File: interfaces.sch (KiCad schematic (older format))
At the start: 11 parts

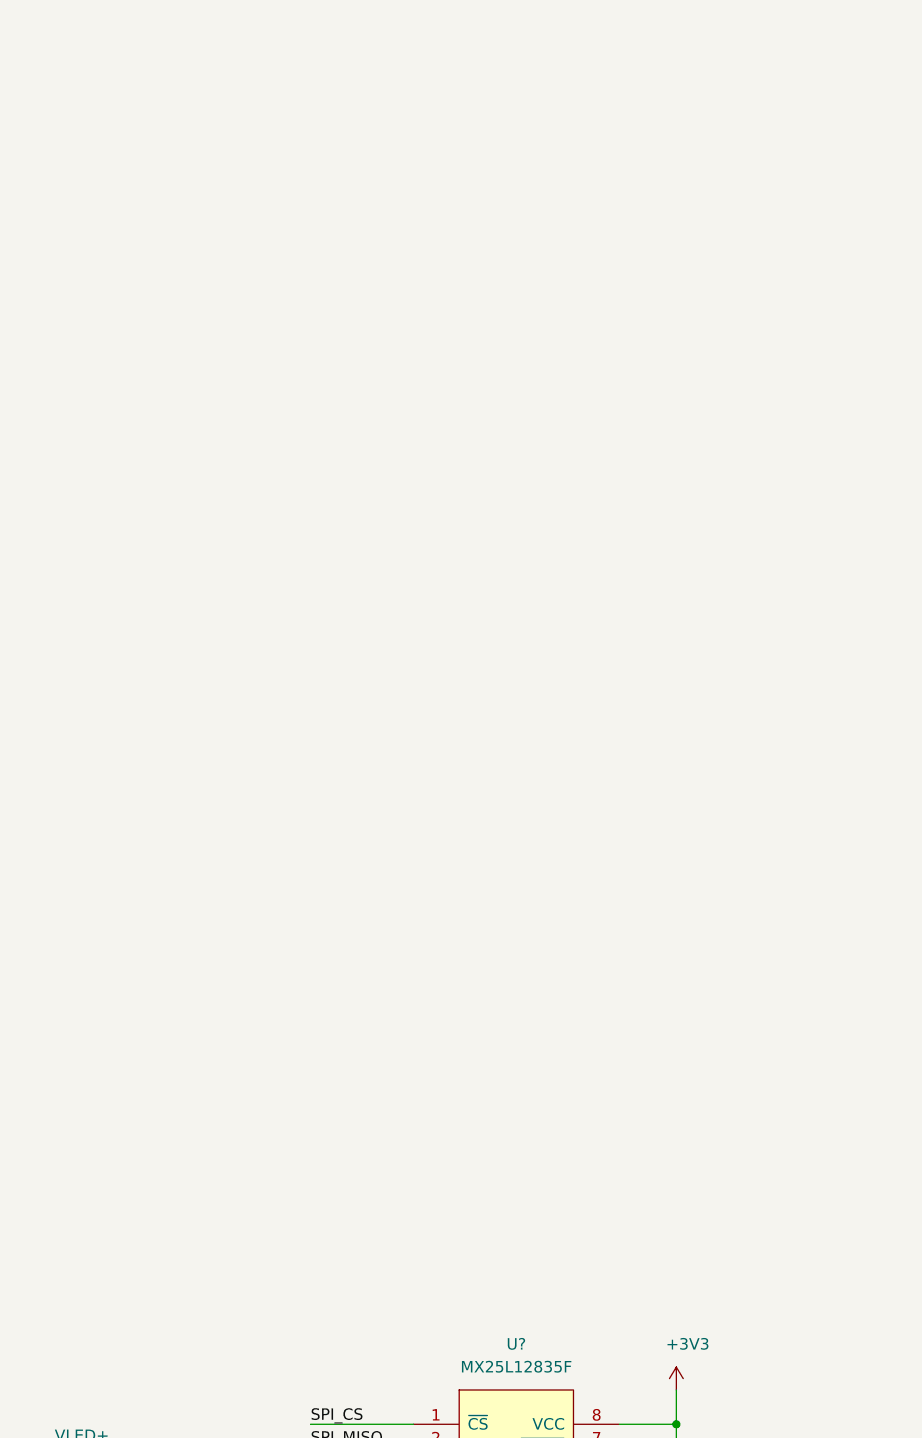
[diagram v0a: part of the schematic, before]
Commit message: update,
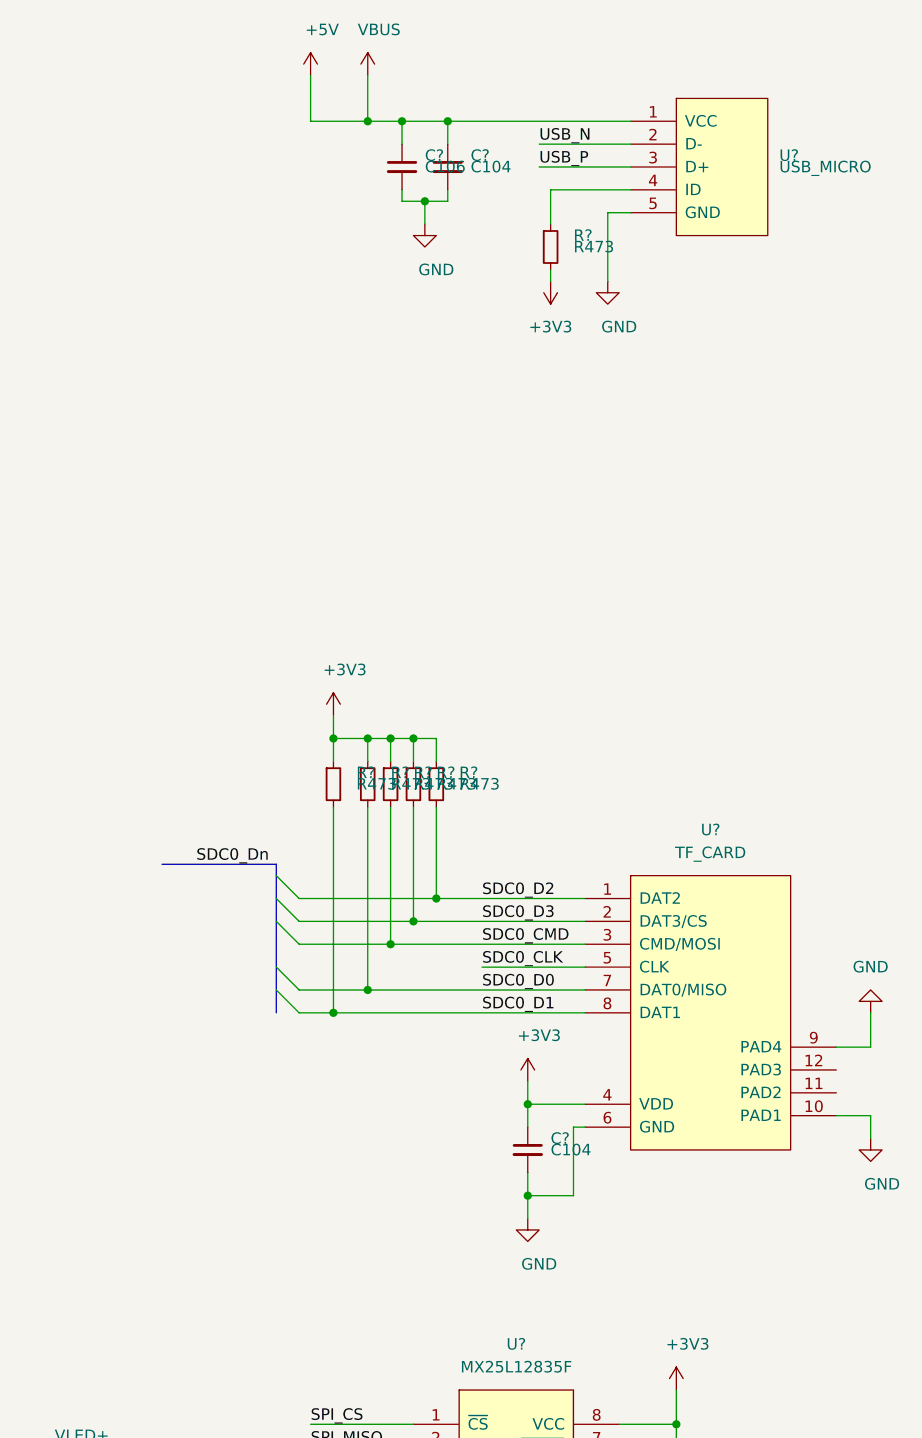
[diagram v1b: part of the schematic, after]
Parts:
- added C? (x2): C104, symbol taobao-c:C104
- added C?: C106, symbol taobao-c:C106
- added R? (x6): R473, symbol taobao-r:R473
- added U?: TF_CARD, symbol taobao-components:TF_CARD
- added U?: USB_MICRO, symbol taobao-components:USB_MICRO
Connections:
- net labels added: SDC0_CLK, SDC0_CMD, SDC0_D0, SDC0_D1, SDC0_D2, SDC0_D3, SDC0_Dn, USB_N, USB_P, VBUS
- wire segments 108 -> 166

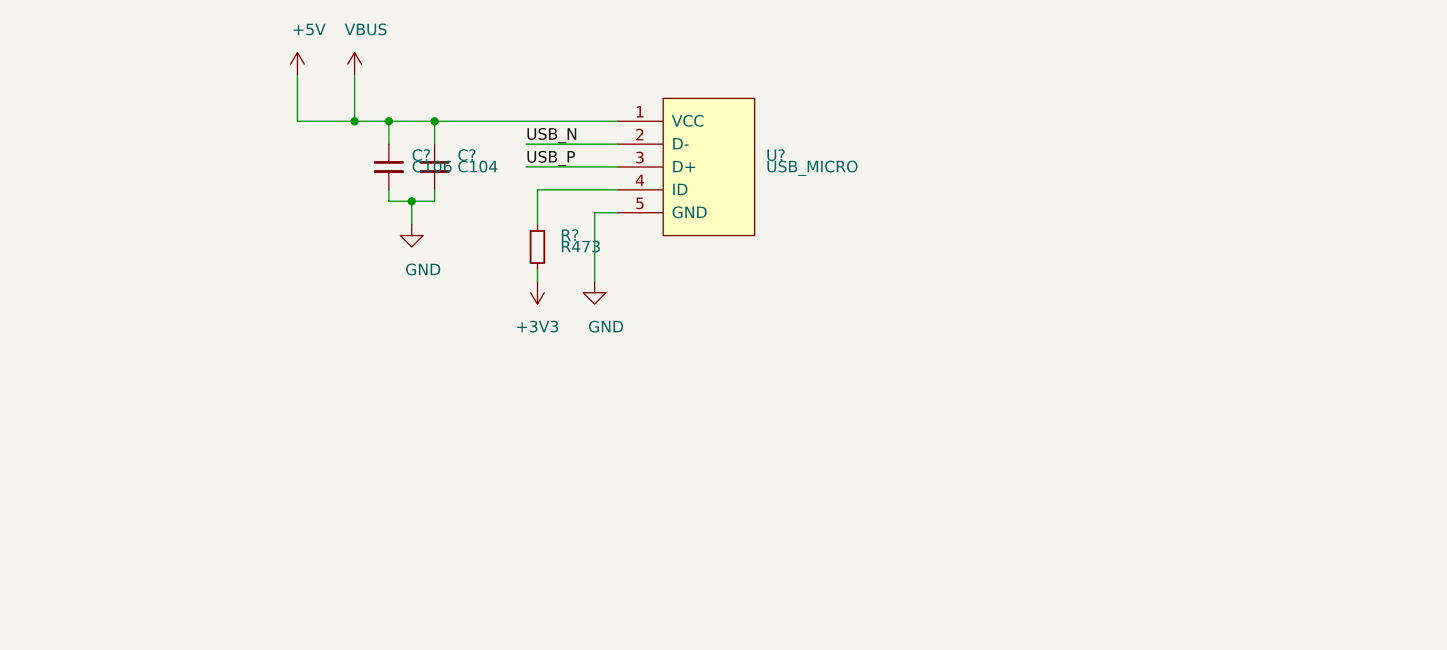
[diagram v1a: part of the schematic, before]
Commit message: update,
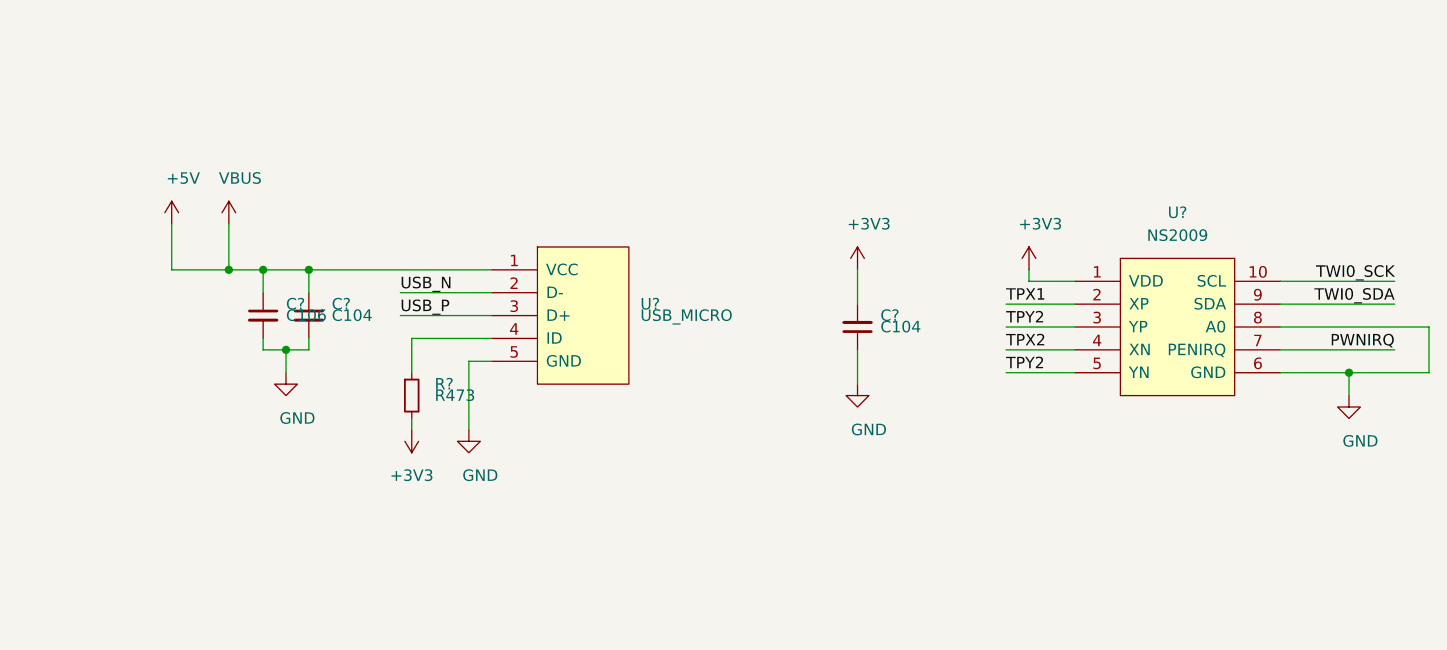
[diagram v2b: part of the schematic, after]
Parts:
- added C?: C104, symbol taobao-c:C104
- added U?: NS2009, symbol taobao-components:NS2009
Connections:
- net labels added: PWNIRQ, TWI0_SCK, TWI0_SDA
- wire segments 166 -> 182
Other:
- moved on the sheet: C?, R?, U?
